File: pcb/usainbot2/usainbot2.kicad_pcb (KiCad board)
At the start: 2 copper layers, 147.3 x 132.1 mm, 13 parts, among them J1 BT_MOD, J2 QTR1-L, J3 QTR1-R, J4 QTR8, J5 SWITCH, M1 Conn_01x02_Male, M2 Conn_01x02_Male, SW1 BTN1, SW2 BTN2, U1 TB6612FNG_breakout

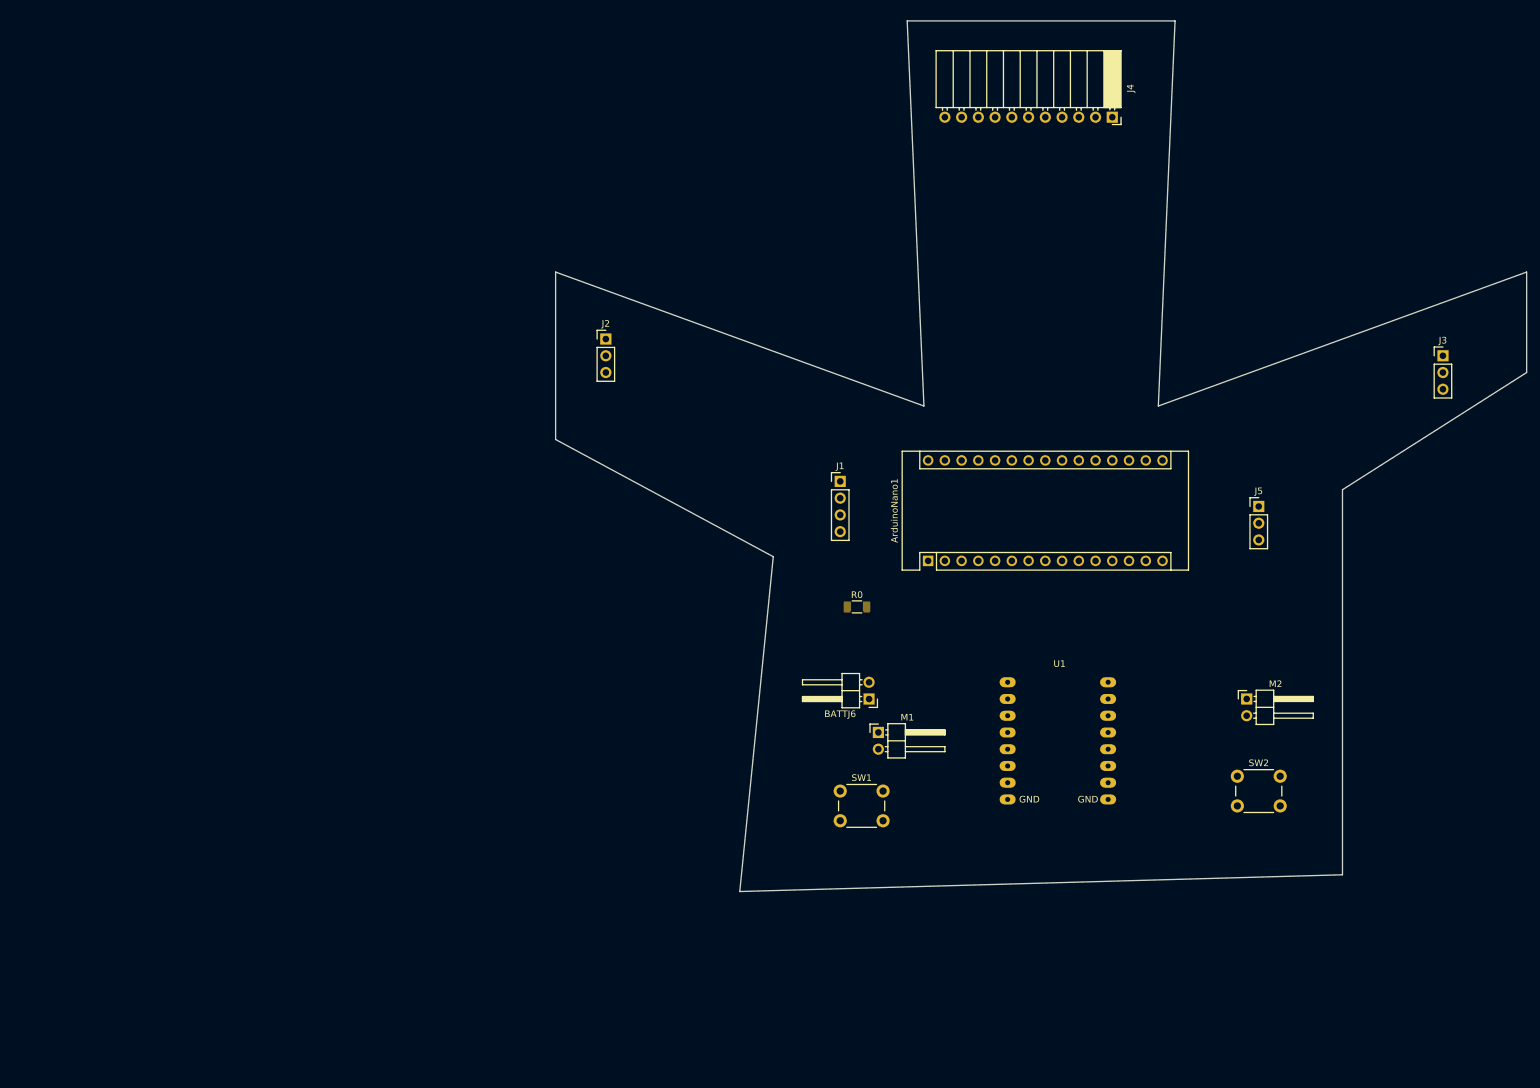
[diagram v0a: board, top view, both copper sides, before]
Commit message: update pcb, falta rutear
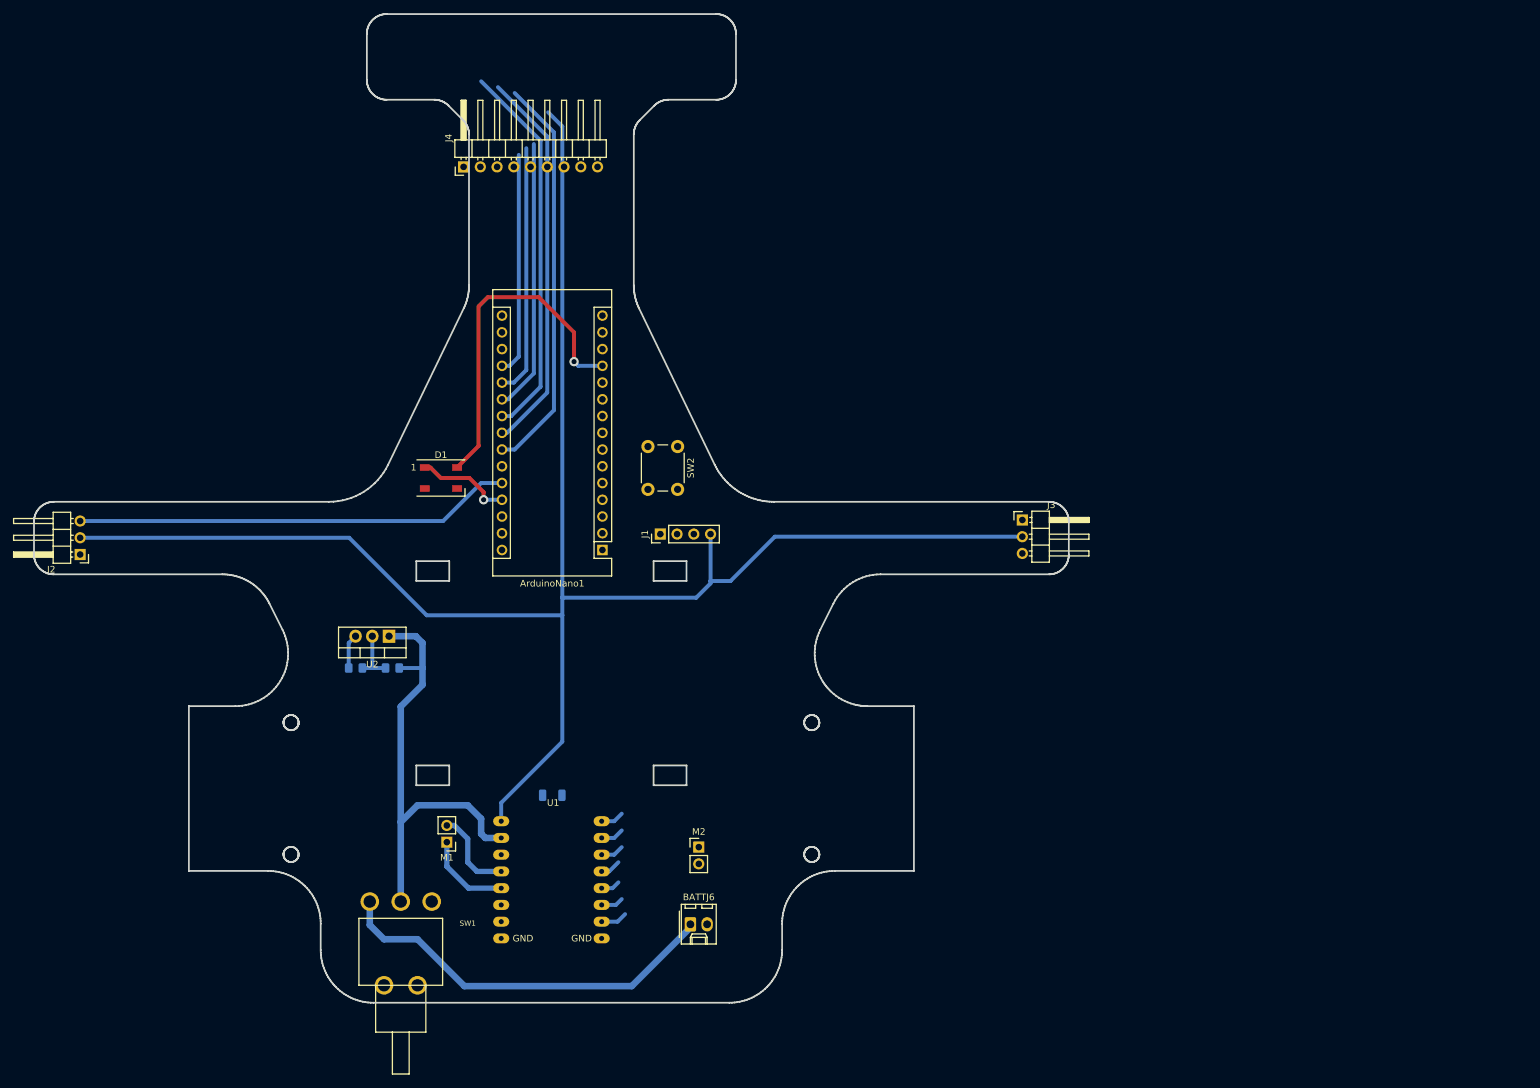
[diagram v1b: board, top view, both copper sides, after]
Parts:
- removed J5: SWITCH, Connector_PinHeader_2.54mm:PinHeader_1x03_P2.54mm_Vertical
- added C1: C, Capacitor_SMD:C_0805_2012Metric_Pad1.18x1.45mm_HandSolder, B.Cu at (74.3, 121.0)
- added C2: C, Capacitor_SMD:C_0805_2012Metric_Pad1.18x1.45mm_HandSolder, B.Cu at (68.7, 121.0)
- added D1: WS2812B, LED_SMD:LED_WS2812B_PLCC4_5.0x5.0mm_P3.2mm, F.Cu at (81.7, 92.2)
- added U2: LM7805_TO220, Package_TO_SOT_THT:TO-220-3_Vertical, F.Cu at (73.8, 116.2)
- BATTJ6: footprint Connector_PinHeader_2.54mm:PinHeader_1x02_P2.54mm_Horizontal -> Connector_Molex:Molex_KK-254_AE-6410-02A_1x02_P2.54mm_Vertical
- J2, J3: footprint Connector_PinHeader_2.54mm:PinHeader_1x03_P2.54mm_Vertical -> Connector_PinHeader_2.54mm:PinHeader_1x03_P2.54mm_Horizontal
- J4: value QTR8 -> QTR-6A; footprint Connector_PinSocket_2.54mm:PinSocket_1x11_P2.54mm_Horizontal -> Connector_PinHeader_2.54mm:PinHeader_1x09_P2.54mm_Horizontal
- M1, M2: footprint Connector_PinHeader_2.54mm:PinHeader_1x02_P2.54mm_Horizontal -> Connector_PinHeader_2.54mm:PinHeader_1x02_P2.54mm_Vertical
- R0: moved to B.Cu
- SW1: value BTN1 -> SW_SPDT; footprint Button_Switch_THT:SW_PUSH_6mm -> usainbot:TOGGLE_RA
- moved J4 98.7 mm to (85.1, 45.0), turned to 90 degrees
- moved SW2 98.6 mm to (117.6, 87.4), turned to -90 degrees
- moved J2 86.2 mm to (26.9, 103.8), turned to 180 degrees
- moved M2 86.1 mm to (120.8, 148.2)
- moved U1 79.7 mm to (98.4, 153.2)
- moved SW1 72.9 mm to (75.6, 169.2)
- moved J3 68.5 mm to (169.9, 98.6)
- moved M1 67.6 mm to (82.6, 147.5), turned to 180 degrees
- moved R0 54.3 mm to (98.6, 140.3), turned to 180 degrees
- moved ArduinoNano1 49.4 mm to (106.2, 103.1), turned to 180 degrees
- moved BATTJ6 43.6 mm to (119.5, 159.9), turned to 0 degrees
- moved J1 28.4 mm to (114.9, 100.7), turned to 90 degrees
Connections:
- ArduinoNano1 pad 10: /BTN1 -> /BTN2
- ArduinoNano1 pad 11: /BTN2 -> unconnected-(ArduinoNano1-Pad11)
- ArduinoNano1 pad 12: unconnected-(ArduinoNano1-Pad12) -> Net-(ArduinoNano1-Pad12)
- ArduinoNano1 pad 25: Net-(ArduinoNano1-Pad25) -> /A6
- ArduinoNano1 pad 26: Net-(ArduinoNano1-Pad26) -> /A7
- ArduinoNano1 pad 27: +5V -> Net-(D1-Pad1)
- ArduinoNano1 pad 5: Net-(ArduinoNano1-Pad5) -> unconnected-(ArduinoNano1-Pad5)
- ArduinoNano1 pad 6: Net-(ArduinoNano1-Pad6) -> unconnected-(ArduinoNano1-Pad6)
- J2 pad 3: Net-(ArduinoNano1-Pad5) -> /A7
- J3 pad 3: Net-(ArduinoNano1-Pad6) -> /A6
- J4 pad 7: Net-(ArduinoNano1-Pad25) -> unconnected-(J4-Pad7)
- J4 pad 8: Net-(ArduinoNano1-Pad26) -> +5V
- J4 pad 9: unconnected-(J4-Pad9) -> GND
- SW1 pad 2: /BTN1 -> VCC
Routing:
- net +5V: track 0.00 -> 276.5 mm
- net VCC: track 0.00 -> 69.3 mm
- net /A7: track 0.00 -> 66.4 mm
- net Net-(ArduinoNano1-Pad24): track 0.00 -> 60.9 mm
- net Net-(BATTJ6-Pad1): track 0.00 -> 60.2 mm
- net Net-(ArduinoNano1-Pad23): track 0.00 -> 58.8 mm
- net Net-(ArduinoNano1-Pad22): track 0.00 -> 57.8 mm
- net Net-(ArduinoNano1-Pad12): track 0.00 -> 52.1 mm, vias 0 -> 1
- net Net-(ArduinoNano1-Pad21): track 0.00 -> 41.3 mm
- net Net-(ArduinoNano1-Pad20): track 0.00 -> 38.1 mm
- net Net-(ArduinoNano1-Pad19): track 0.00 -> 33.7 mm
- net Net-(D1-Pad1): track 0.00 -> 14.4 mm, vias 0 -> 1
- net Net-(M1-Pad1): track 0.00 -> 13.3 mm
- net Net-(M1-Pad2): track 0.00 -> 13.2 mm
- net GND: track 0.00 -> 8.44 mm
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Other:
- board size 147.3 x 132.1 mm -> 157 x 150 mm
- rule pad_to_mask_clearance: 0 -> 0.0508
